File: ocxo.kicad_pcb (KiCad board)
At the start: 2 copper layers, 50 x 50 mm, 297 parts, among them J1 Conn_01x02, J2 Conn_01x01, J3 Conn_Coaxial, J5 Conn_01x01, J6 Conn_01x01, Q1 ENE3311 OCXO, U1 KA78M05_TO252, U2 LM4140

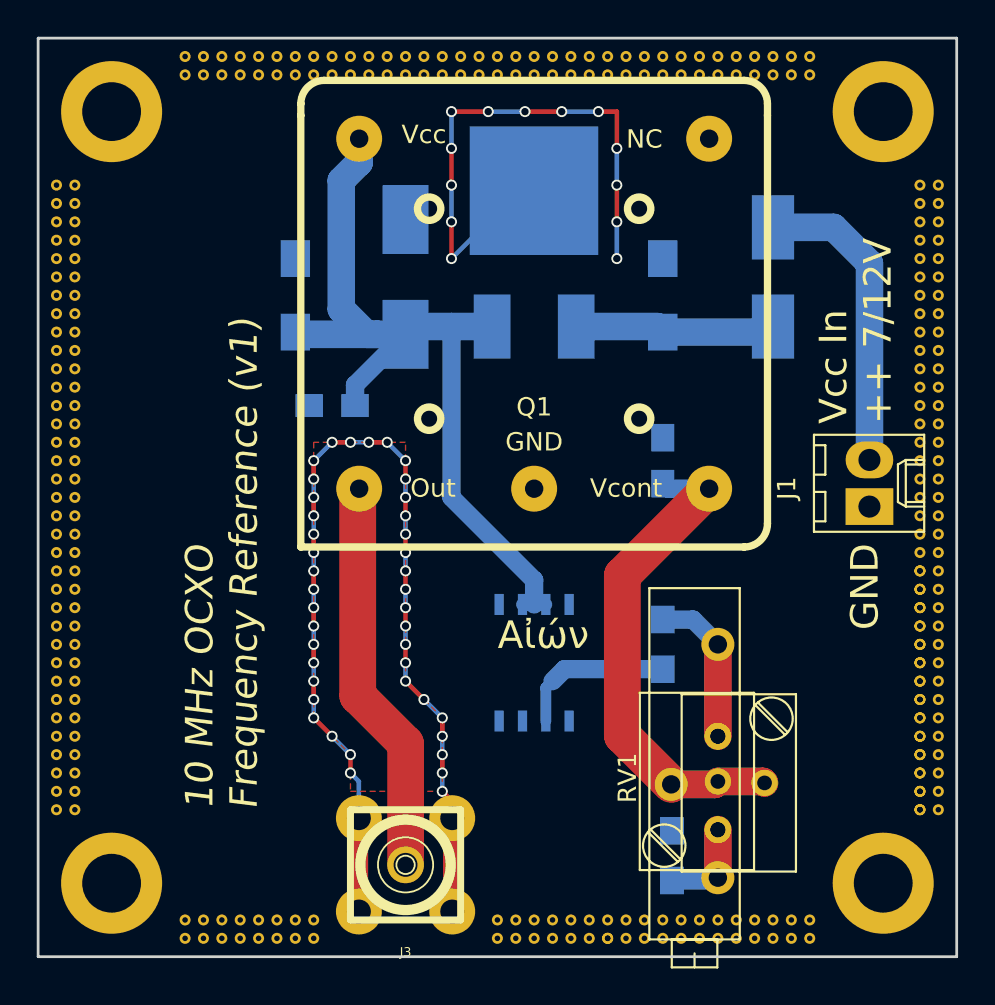
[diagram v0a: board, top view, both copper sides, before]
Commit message: new iBom
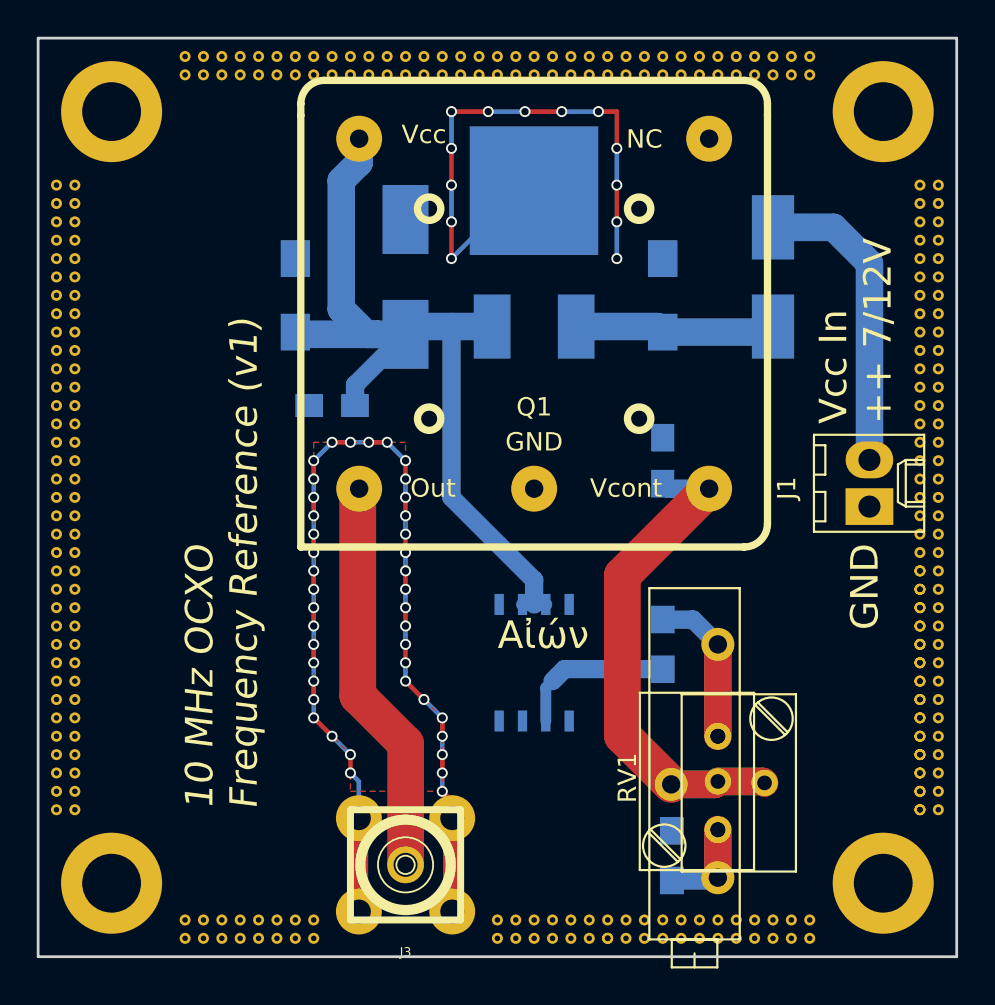
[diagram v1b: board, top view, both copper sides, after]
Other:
- net class Default removed
